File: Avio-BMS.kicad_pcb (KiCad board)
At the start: 2 copper layers, 80 x 80 mm, 107 parts, among them J1 MainBattery, J2 5077CR-16SMC2-BK-TR, J3 SubBattery, J4 Conn_01x03_Pin, J5 Conn_01x03_Pin, J6 +3.3V, J7 +6V, J8 +3.3V, J9 +6V, Q1 Si2333DDS-T1-GE3, Q2 Si2333DDS-T1-GE3, Q3 IRF7324, Q4 IRF7324, U1 LTC4088EDE-TRPBF, U2 LTC4417CGN, U3 TPS63021DSJR, U4 TPS61088RHLR

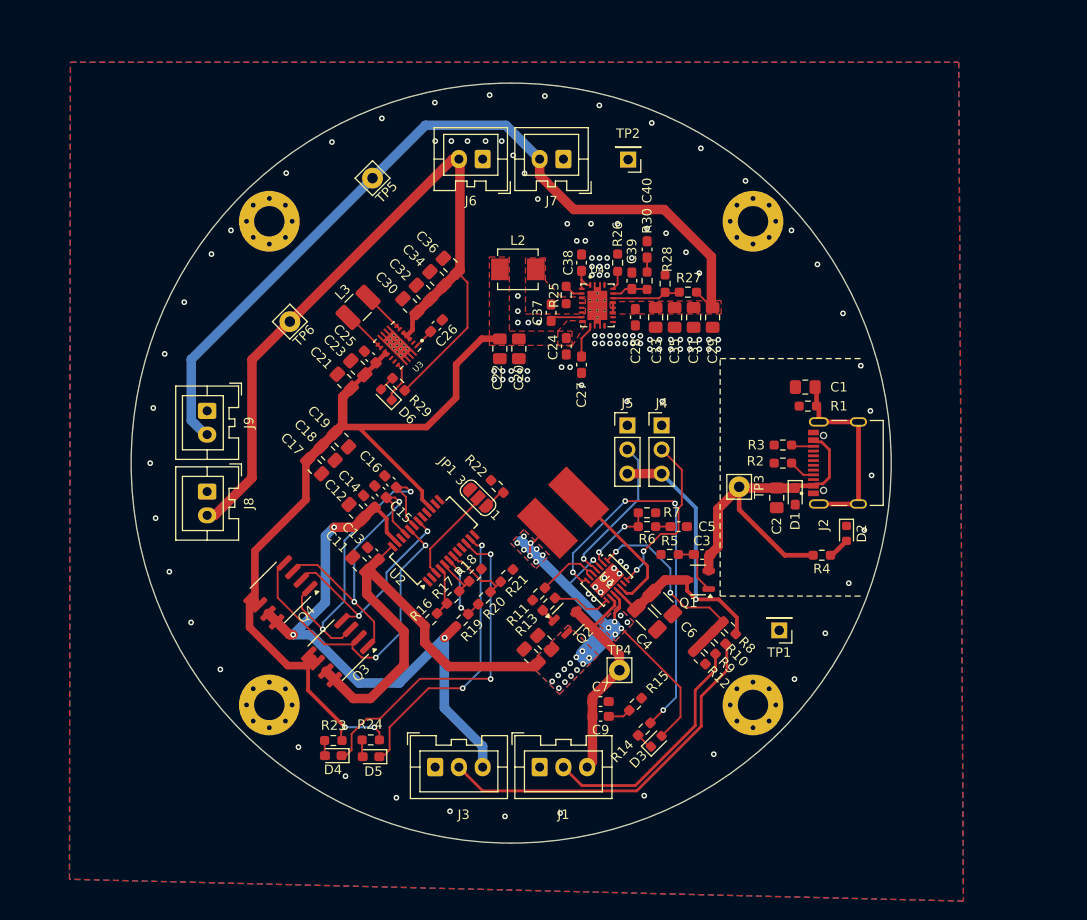
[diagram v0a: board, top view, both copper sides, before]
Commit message: update
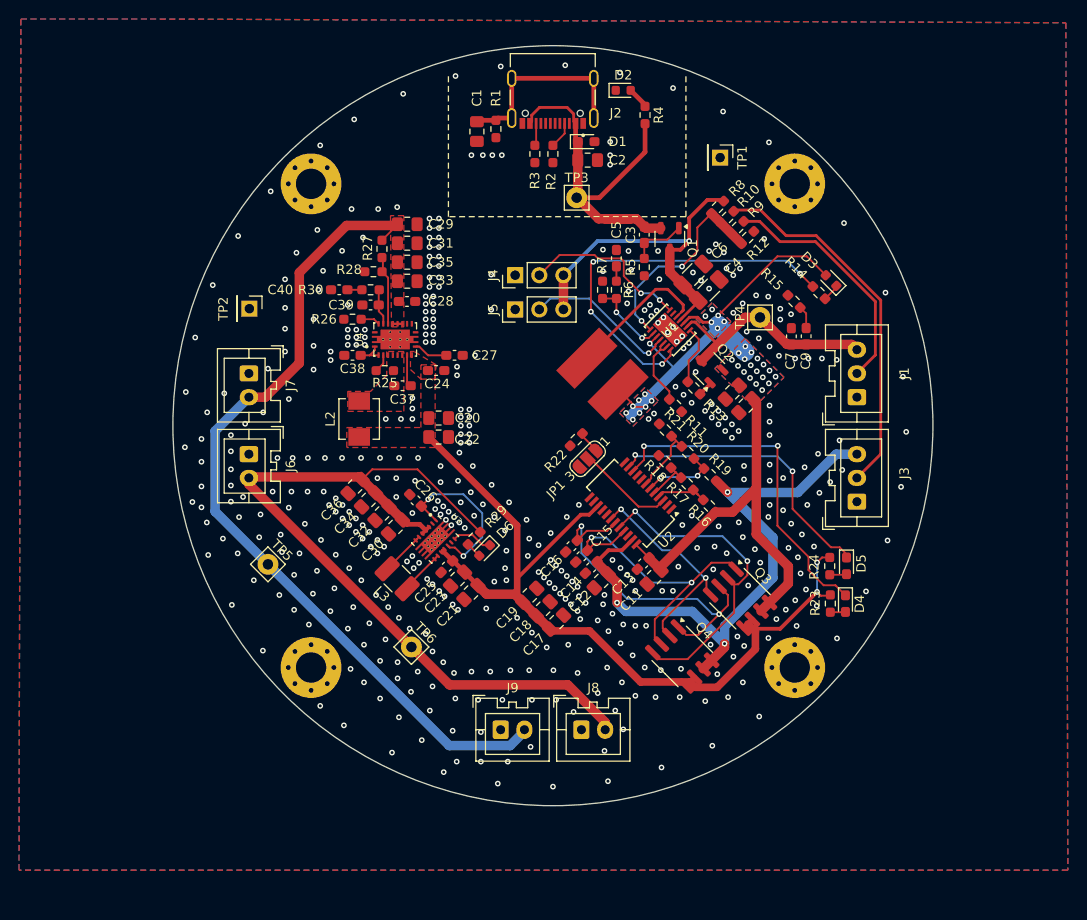
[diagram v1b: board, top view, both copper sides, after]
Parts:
- moved D4 56.2 mm to (188.1, 104.5), turned to -90 degrees
- moved REF** 55.4 mm to (182.8, 111.2), turned to -45 degrees
- moved REF** 55.0 mm to (182.8, 60.3), turned to -45 degrees
- moved R23 54.3 mm to (186.5, 104.5), turned to 90 degrees
- moved D5 53.9 mm to (188.3, 100.5), turned to -90 degrees
- moved J3 52.5 mm to (189.3, 93.8), turned to 90 degrees
- moved D2 52.2 mm to (164.7, 50.5), turned to 0 degrees
- moved D3 51.9 mm to (186.6, 70.5), turned to 135 degrees
- moved R24 51.7 mm to (186.5, 100.6), turned to 90 degrees
- moved J1 51.3 mm to (189.3, 82.8), turned to 90 degrees
- moved TP1 50.1 mm to (175.0, 57.6), turned to -90 degrees
- moved R4 49.9 mm to (167.0, 53.1), turned to -90 degrees
- moved R14 49.5 mm to (185.4, 71.8), turned to 135 degrees
- moved REF** 47.2 mm to (131.9, 111.2), turned to -45 degrees
- moved J8 46.7 mm to (160.3, 117.8), turned to 0 degrees
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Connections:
- J5 pad 2: /Li-ionBatteryCharger,PowerPath/D1 -> /Li-ionBatteryCharger,PowerPath/D2
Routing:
- net /Li-ionBatteryCharger,PowerPath/D2: track 0.00 -> 16.3 mm, vias 0 -> 1
- net (no net): track 16.3 -> 0.00 mm, vias 1 -> 0
- net Net-(U3-EN): track 2.13 -> 17.3 mm, vias 0 -> 2
- net V1: track 94.6 -> 87.8 mm, vias 27 -> 33
- net VCC: track 99.2 -> 97.2 mm
- net Net-(Q3B-S2): track 35.1 -> 35.7 mm
- net GND: vias 125 -> 449
